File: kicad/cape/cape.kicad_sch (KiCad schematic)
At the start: 13 parts, among them M1 HSR-2648CR, P1 BeagleBone_Black_Header, P2 BeagleBone_Black_Header, SW1 L101011_SPST, U1 L298, U2 BNO055, U3 BMP390, U4 S13V10FS

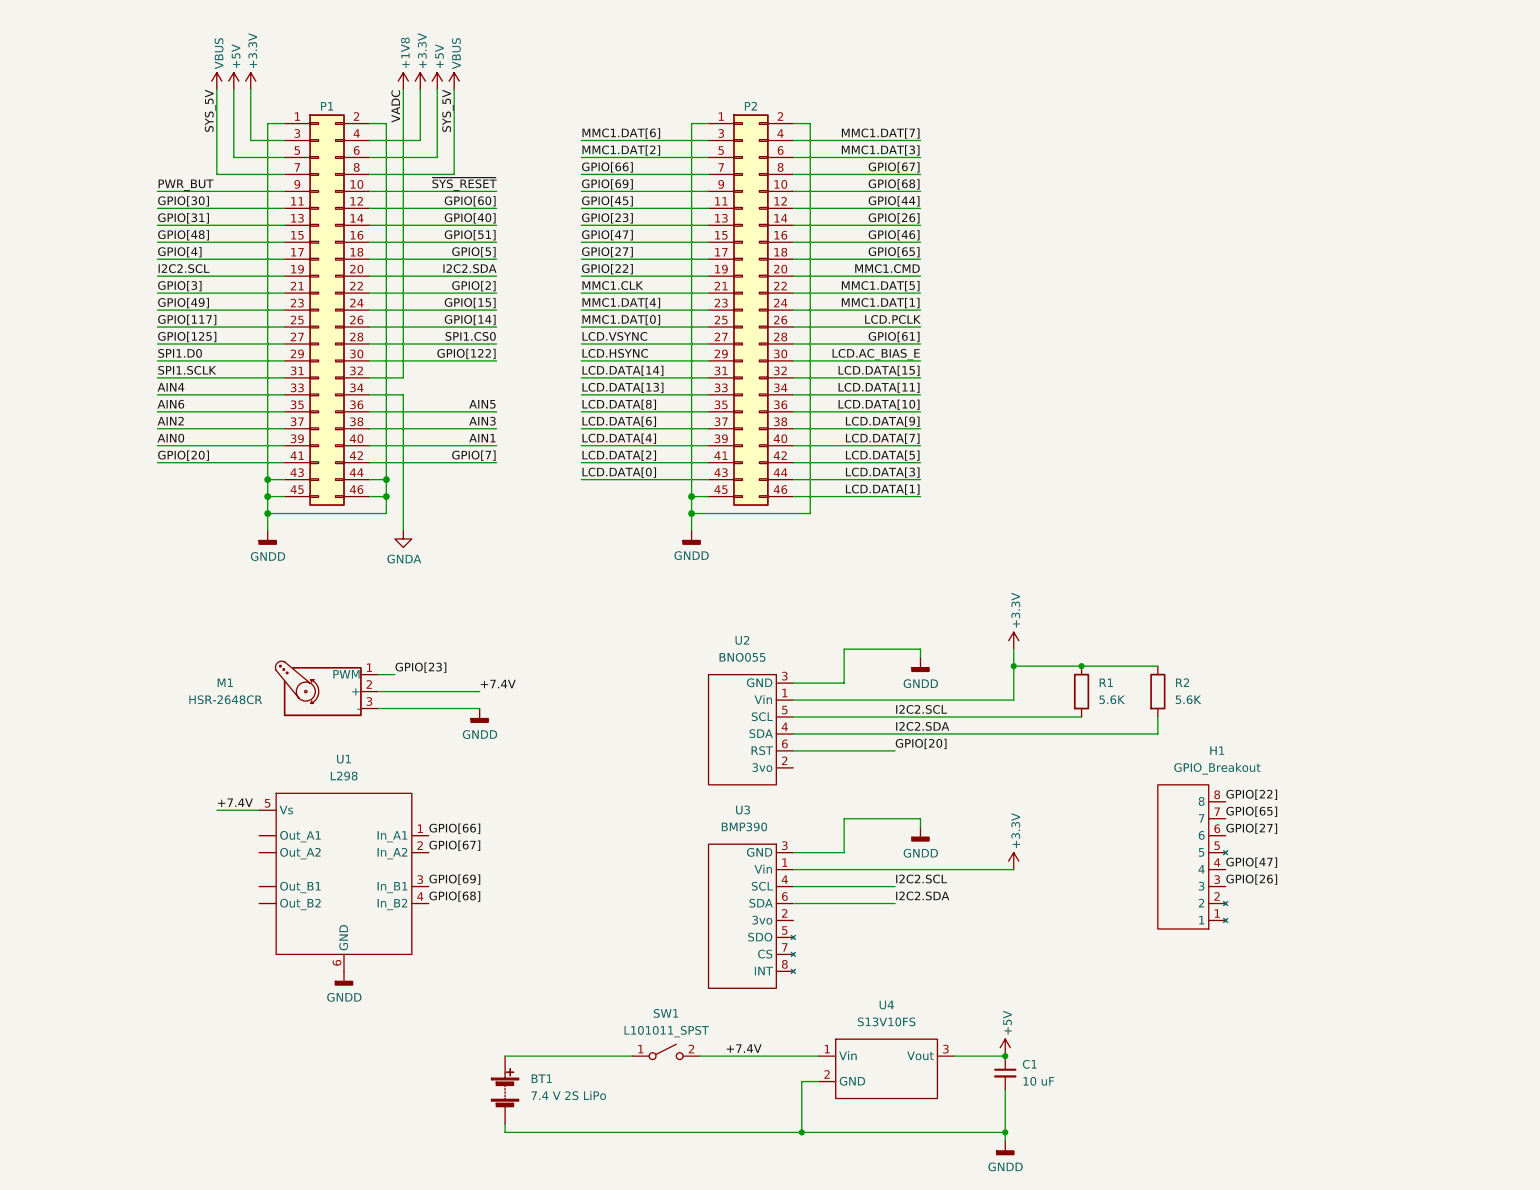
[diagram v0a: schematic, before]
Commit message: Cape v 1.2
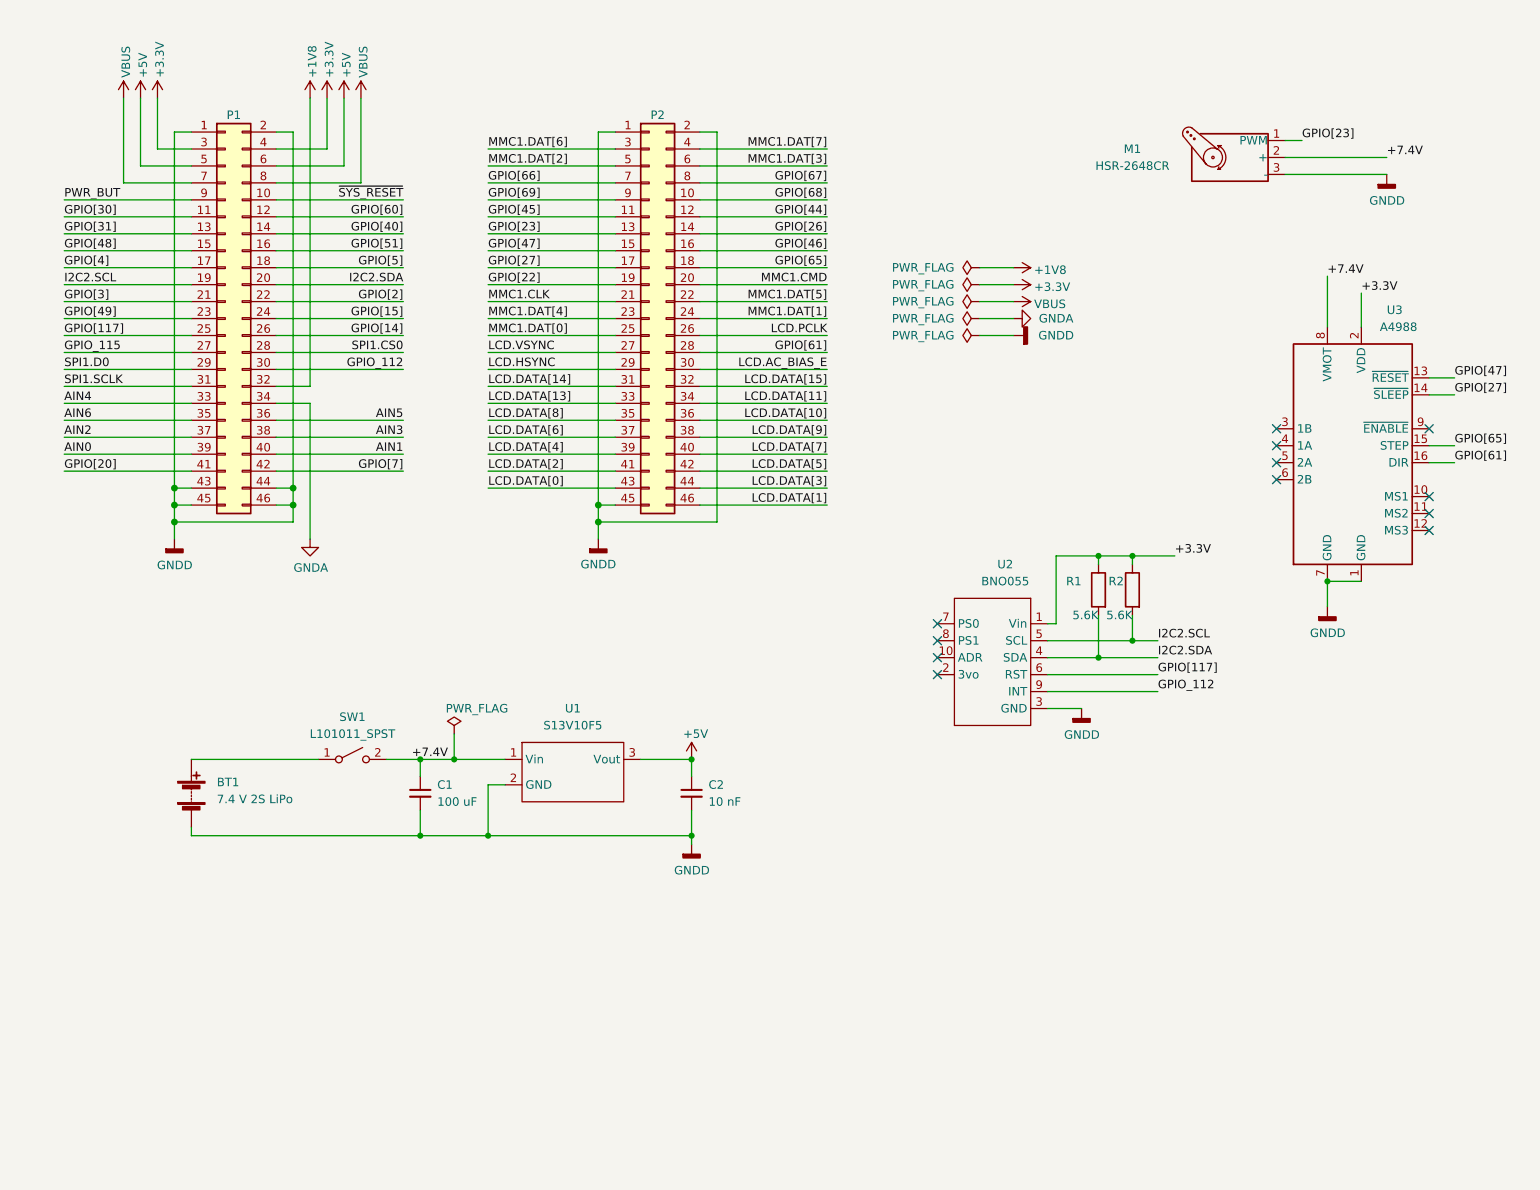
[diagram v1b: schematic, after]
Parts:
- removed H1: GPIO_Breakout, Connector_PinHeader_2.54mm:PinHeader_1x08_P2.54mm_Vertical, symbol payload_symbol_library:GPIO_Breakout
- removed U1: L298, Connector_PinHeader_2.54mm:PinHeader_1x06_P2.54mm_Vertical, symbol payload_symbol_library:L298
- removed U3: BMP390, payload_footprint_library:BMP390, symbol payload_symbol_library:BMP390
- added C1: 100 uF, Capacitor_THT:C_Radial_D10.0mm_H16.0mm_P5.00mm, symbol Device:C_Small
- added U3: A4988, payload_footprint_library:Pololu_Breakout-16_15.2x20.3mm, symbol payload_symbol_library:A4988
- C2: renamed from C1; value 10 uF -> 10 nF; footprint Capacitor_THT:C_Radial_D10.0mm_H16.0mm_P5.00mm -> Capacitor_THT:C_Disc_D10.0mm_W2.5mm_P5.00mm
- M1: footprint Connector_PinHeader_2.54mm:PinHeader_1x03_P2.54mm_Vertical -> Connector_PinSocket_2.54mm:PinSocket_1x03_P2.54mm_Vertical
- SW1: footprint payload_footprint_library:SPST -> payload_footprint_library:SW_L101011MS02Q
- U1: renamed from U4; value S13V10FS -> S13V10F5; symbol payload_symbol_library:S13V10FS -> payload_symbol_library:S13V10F5
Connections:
- net +3.3V: now also U3.2 (VDD)
- net +7.4V: now also C1.1, U3.8 (VMOT)
- net GNDD: now also C1.2, U3.1 (GND), U3.7 (GND)
- net GPIO[117]: now also U2.6 (RST)
- net GPIO[20]: no longer U2.6 (RST)
- net GPIO[27]: now also U3.14 (~{SLEEP})
- net GPIO[47]: now also U3.13 (~{RESET})
- net GPIO[61]: now also U3.16 (DIR)
- net GPIO[65]: now also U3.15 (STEP)
- net I2C2.SCL: now also R2.2; no longer R1.2
- net I2C2.SDA: now also R1.2; no longer R2.2
- net GPIO[122] renamed GPIO_112
- net GPIO_112: now also U2.9 (INT)
- net GPIO[125] renamed GPIO_115
- no-connect marks 0 -> 12
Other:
- moved on the sheet: BT1, C2, M1, P1, P2, SW1, U1

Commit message: Cape 1.3, Main 1.7
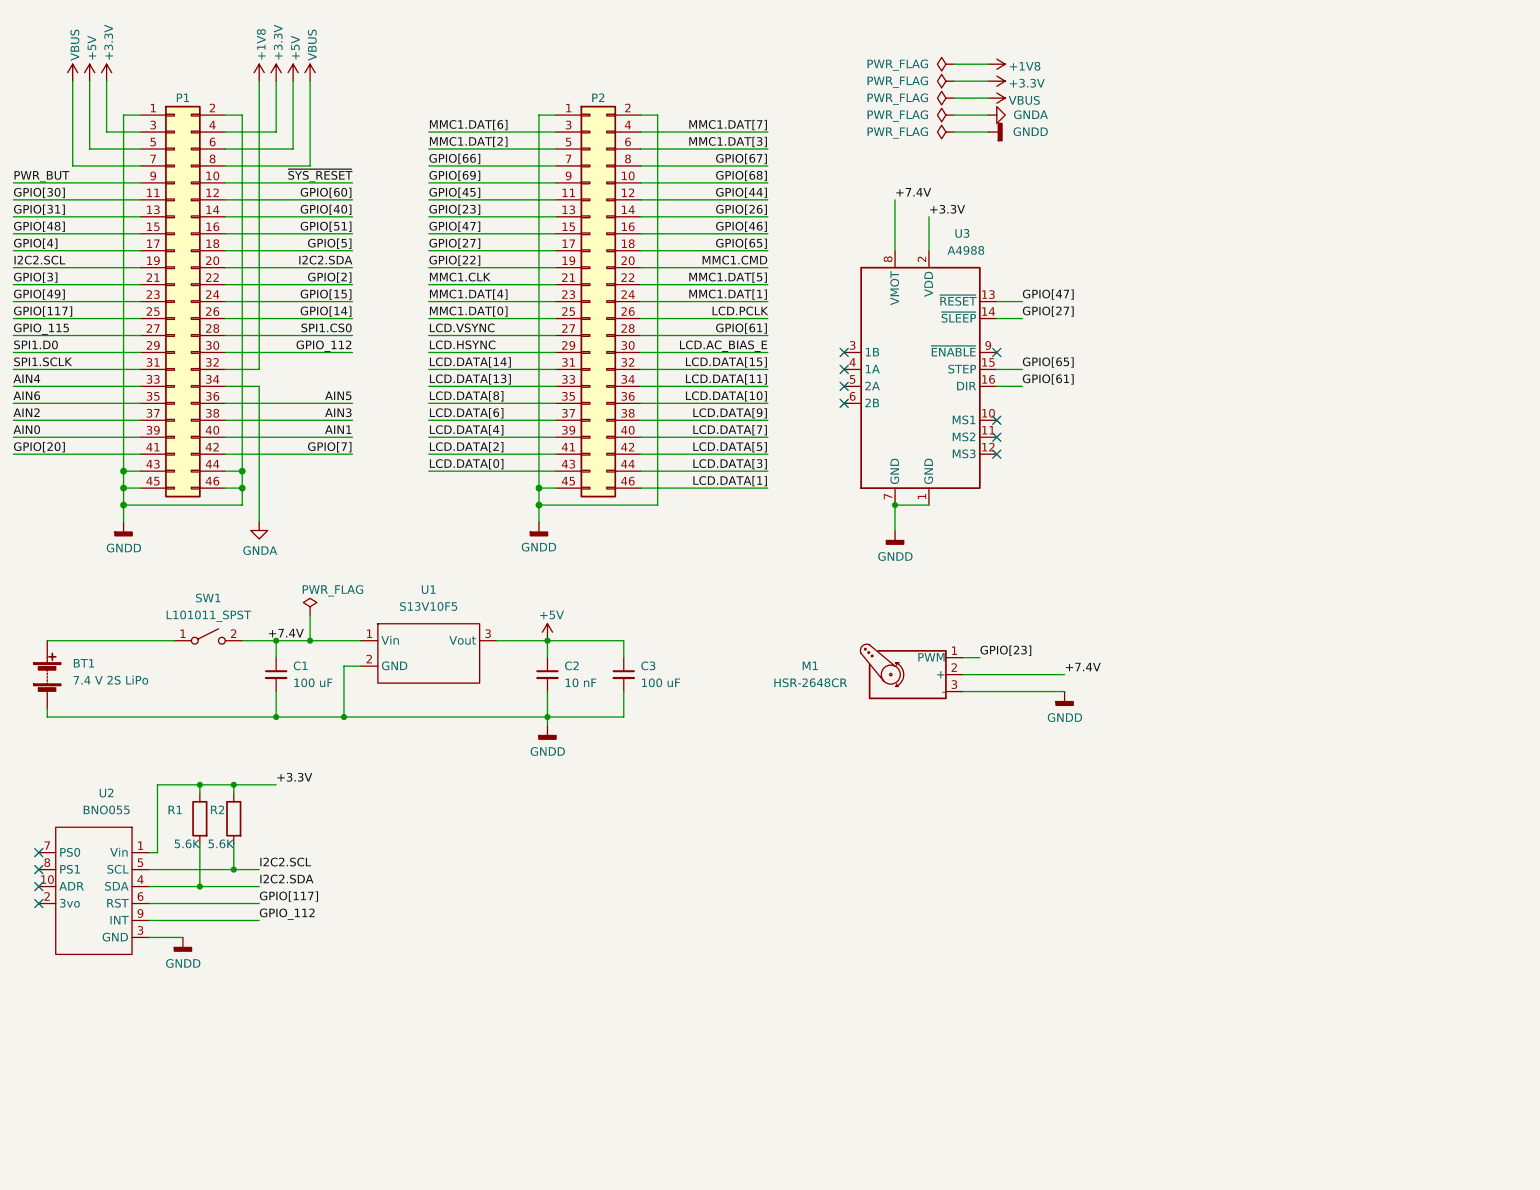
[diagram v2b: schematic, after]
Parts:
- added C3: 100 uF, Capacitor_THT:C_Radial_D10.0mm_H16.0mm_P5.00mm, symbol Device:C_Small
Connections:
- net +5V: now also C3.1
- net GNDD: now also C3.2
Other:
- moved on the sheet: BT1, C1, C2, M1, P1, P2, R1, R2, SW1, U1, U2, U3
